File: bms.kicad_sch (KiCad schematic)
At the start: 36 parts, among them IC1 BQ25303JRTER, J1 10118192-0002LF, J4 691213710002, J4 Conn_01x01_Pin, J5 Conn_01x01_Pin, U1 TPS63001DRCR, U5 ADP1109AN-12, U6 ADP1109AN-12, U8 MIC2876-5.0YMT-TR

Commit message: routing
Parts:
- 1uH1: footprint VLS252012HBX-1R0M-1:IND_VLS252012HBX-1R0M-1 -> 1 uH Ind:IND_VLS252012HBX-1R0M-1
- C14, C15, C19, C20: footprint (none) -> Capacitor_SMD:C_0603_1608Metric_Pad1.08x0.95mm_HandSolder
- D1: footprint 0603 LED:LEDC1608X35N -> 0603 LED:LED_150060GS75000_WRE-M
- IC1: footprint bq2530rter:RTE0016C -> BQ2530:RTE0016C_NV
- J1: footprint Micro USB:AMPHENOL_10118192-0002LF -> Micro USB:AMPHENOL_10118192-0001LF
- J4: footprint 691213710002:691213710002 -> Connector_PinSocket_2.54mm:PinSocket_1x02_P2.54mm_Horizontal
- L1: footprint 1UH -IND:IND_VLS252012HBX-1R0M-1 -> 1 uH Ind:IND_VLS252012HBX-1R0M-1
- L2: footprint 2.2UH-IND:IND_VLS4012ET-2R2M -> 3.3v Power Ind:VLS4012
- L3, L4: footprint (none) -> 12v Power Ind:46473C
- U1: footprint tps63001:DRC0010J -> TPS63001:TPS63002DRCT
- U5, U6: footprint N_8_ADI -> ADP1109:N_8_ADI
- U8: footprint UDFN8_2X2_MCH -> 5v Converter:UDFN8_2X2_MCH-L
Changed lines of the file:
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@@
       (effects (font (size 1.27 1.27)) (justify left))
     )
-    (property "Footprint" "" (at 262.5852 139.7 0)
+    (property "Footprint" "Capacitor_SMD:C_0603_1608Metric_Pad1.08x0.95mm_HandSolder" (at 262.5852 139.7 0)
       (effects (font (size 1.27 1.27)) hide)
     )
@@
       (effects (font (size 1.27 1.27)))
     )
-    (property "Footprint" "1UH -IND:IND_VLS252012HBX-1R0M-1" (at 235.585 30.48 0)
+    (property "Footprint" "1 uH Ind:IND_VLS252012HBX-1R0M-1" (at 235.585 30.48 0)
       (effects (font (size 1.27 1.27)) hide)
     )
@@
       (effects (font (size 1.27 1.27)) (justify left))
     )
-    (property "Footprint" "" (at 177.4952 140.97 0)
+    (property "Footprint" "Capacitor_SMD:C_0603_1608Metric_Pad1.08x0.95mm_HandSolder" (at 177.4952 140.97 0)
       (effects (font (size 1.27 1.27)) hide)
     )
@@
       (effects (font (size 1.27 1.27)) hide)
     )
-    (property "Footprint" "VLS252012HBX-1R0M-1:IND_VLS252012HBX-1R0M-1" (at 46.99 168.91 0)
+    (property "Footprint" "1 uH Ind:IND_VLS252012HBX-1R0M-1" (at 46.99 168.91 0)
       (effects (font (size 1.27 1.27)) (justify bottom) hide)
     )
@@
       (effects (font (size 1.27 1.27)) (justify right))
     )
-    (property "Footprint" "" (at 116.84 119.38 0)
+    (property "Footprint" "12v Power Ind:46473C" (at 116.84 119.38 0)
       (effects (font (size 1.27 1.27)) hide)
     )
@@
       (effects (font (size 1.27 1.27)) (justify left) hide)
     )
-    (property "Footprint" "691213710002:691213710002" (at 77.47 118.11 0)
+    (property "Footprint" "Connector_PinSocket_2.54mm:PinSocket_1x02_P2.54mm_Horizontal" (at 77.47 118.11 0)
       (effects (font (size 1.27 1.27)) (justify bottom) hide)
     )
@@
       (effects (font (size 1.524 1.524)))
     )
-    (property "Footprint" "N_8_ADI" (at 234.95 133.35 0)
+    (property "Footprint" "ADP1109:N_8_ADI" (at 234.95 133.35 0)
       (effects (font (size 1.27 1.27) italic) hide)
     )
@@
       (effects (font (size 1.27 1.27)))
     )
-    (property "Footprint" "bq2530rter:RTE0016C" (at 234.95 44.45 0)
+    (property "Footprint" "BQ2530:RTE0016C_NV" (at 234.95 44.45 0)
       (effects (font (size 1.27 1.27)) (justify left) hide)
     )
@@
       (effects (font (size 0.254 0.254)))
     )
-    (property "Footprint" "0603 LED:LEDC1608X35N" (at 200.025 63.5 0)
+    (property "Footprint" "0603 LED:LED_150060GS75000_WRE-M" (at 200.025 63.5 0)
       (effects (font (size 1.27 1.27)) (justify bottom) hide)
     )
@@
       (effects (font (size 1.27 1.27)) hide)
     )
-    (property "Footprint" "Micro USB:AMPHENOL_10118192-0002LF" (at 29.21 123.19 0)
+    (property "Footprint" "Micro USB:AMPHENOL_10118192-0001LF" (at 29.21 123.19 0)
       (effects (font (size 1.27 1.27)) (justify bottom) hide)
     )
@@
       (effects (font (size 1.27 1.27)) (justify right))
     )
-    (property "Footprint" "" (at 201.93 118.11 0)
+    (property "Footprint" "12v Power Ind:46473C" (at 201.93 118.11 0)
       (effects (font (size 1.27 1.27)) hide)
     )
@@
       (effects (font (size 1.27 1.27)) (justify left))
     )
-    (property "Footprint" "" (at 129.2352 184.15 0)
+    (property "Footprint" "Capacitor_SMD:C_0603_1608Metric_Pad1.08x0.95mm_HandSolder" (at 129.2352 184.15 0)
       (effects (font (size 1.27 1.27)) hide)
     )
@@
       (effects (font (size 1.524 1.524)))
     )
-    (property "Footprint" "UDFN8_2X2_MCH" (at 59.69 173.99 0)
+    (property "Footprint" "5v Converter:UDFN8_2X2_MCH-L" (at 59.69 173.99 0)
       (effects (font (size 1.27 1.27) italic) hide)
     )
@@
       (effects (font (size 1.524 1.524)))
     )
-    (property "Footprint" "tps63001:DRC0010J" (at 63.5 63.5 0)
+    (property "Footprint" "TPS63001:TPS63002DRCT" (at 63.5 63.5 0)
       (effects (font (size 1.27 1.27) italic) hide)
     )
@@
       (effects (font (size 1.524 1.524)))
     )
-    (property "Footprint" "N_8_ADI" (at 149.86 134.62 0)
+    (property "Footprint" "ADP1109:N_8_ADI" (at 149.86 134.62 0)
       (effects (font (size 1.27 1.27) italic) hide)
     )
@@
       (effects (font (size 1.27 1.27)))
     )
-    (property "Footprint" "2.2UH-IND:IND_VLS4012ET-2R2M" (at 62.865 35.56 0)
+    (property "Footprint" "3.3v Power Ind:VLS4012" (at 62.865 35.56 0)
       (effects (font (size 1.27 1.27)) hide)
     )
@@
       (effects (font (size 1.27 1.27)) (justify right))
     )
-    (property "Footprint" "" (at 33.3248 179.07 0)
-      (effects (font (size 1.27 1.27)) hide)
-    )
+    (property "Footprint" "Capacitor_SMD:C_0603_1608Metric_Pad1.08x0.95mm_HandSolder" (at 33.3248 179.07 0)
+      (effects (font (size 1.27 1.27)) hide)
+    )

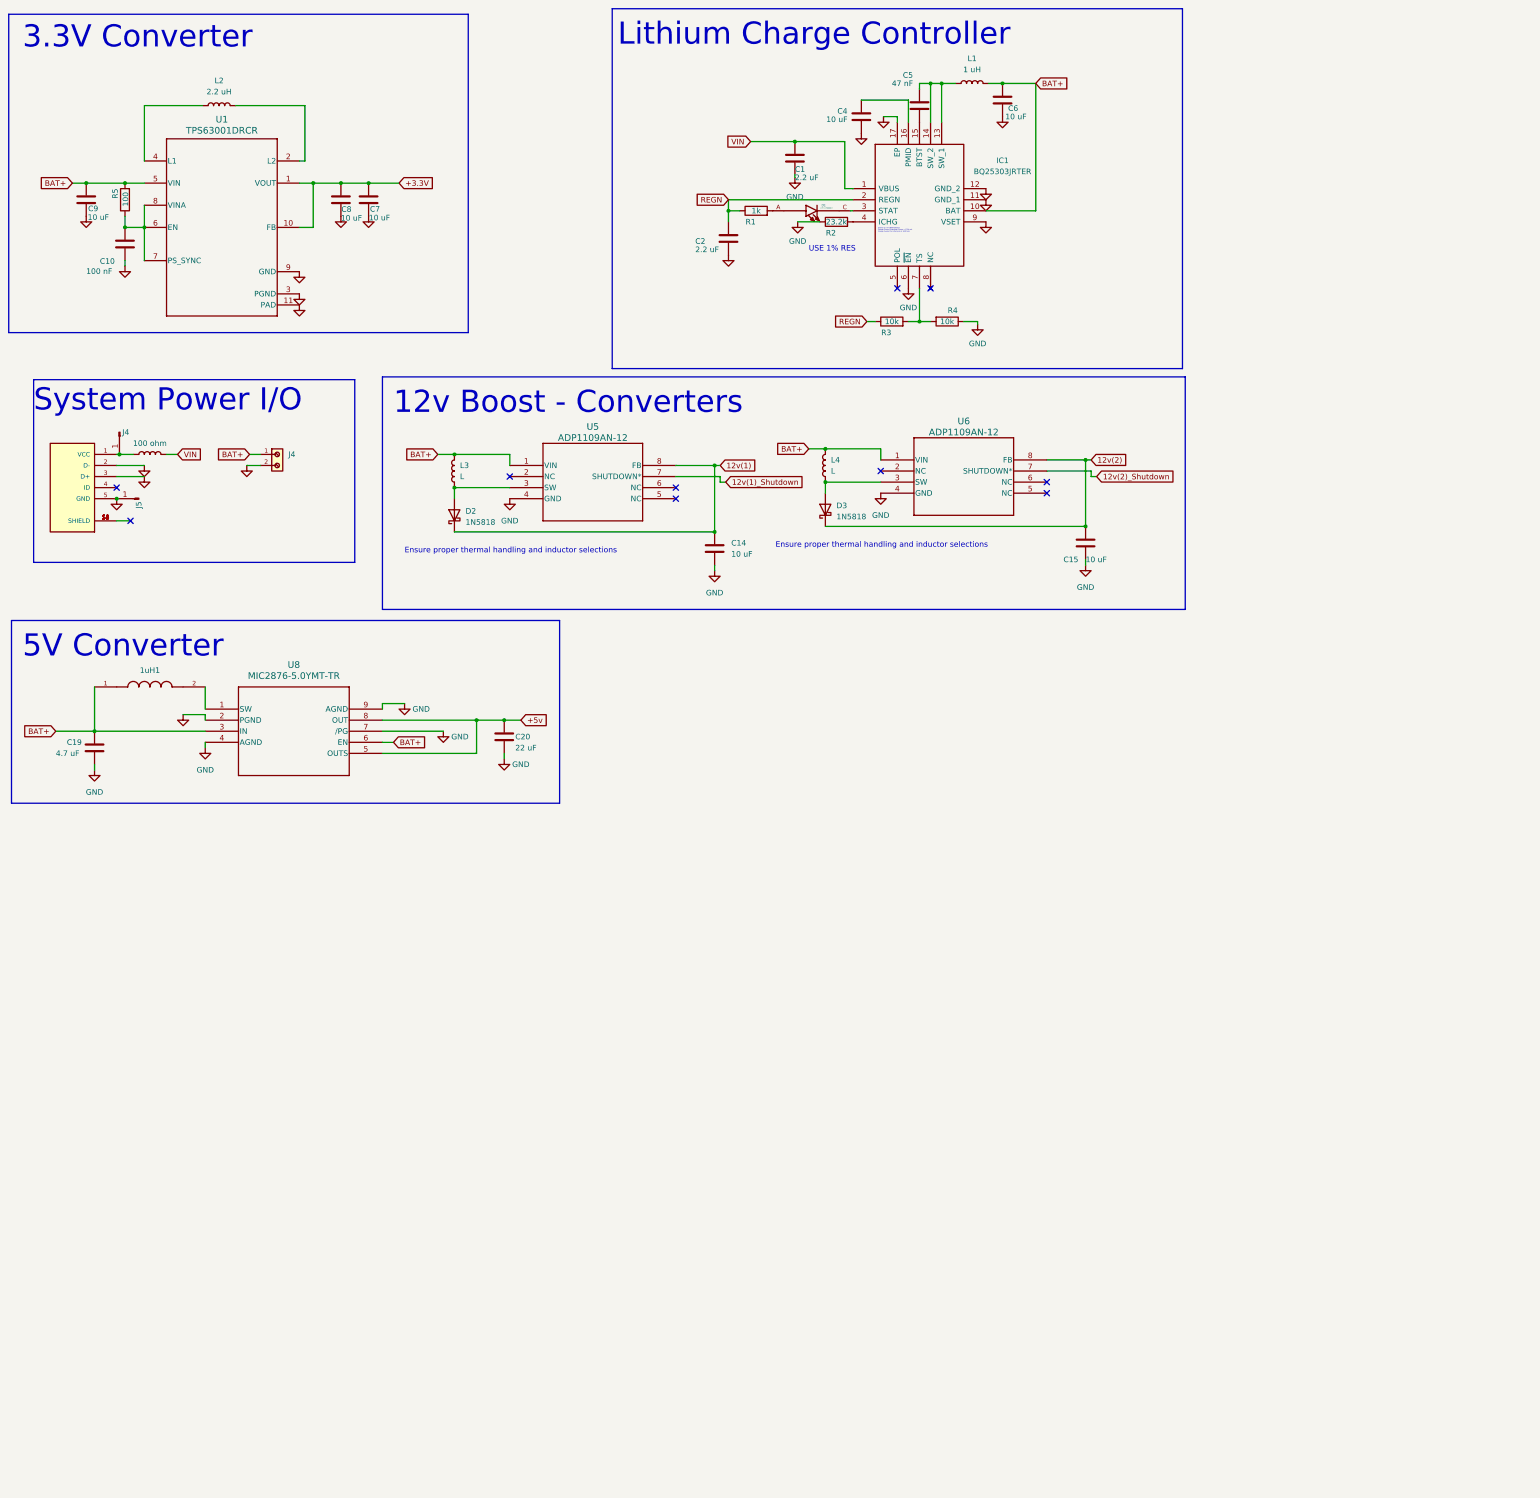
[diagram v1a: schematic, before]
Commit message: Routing begin
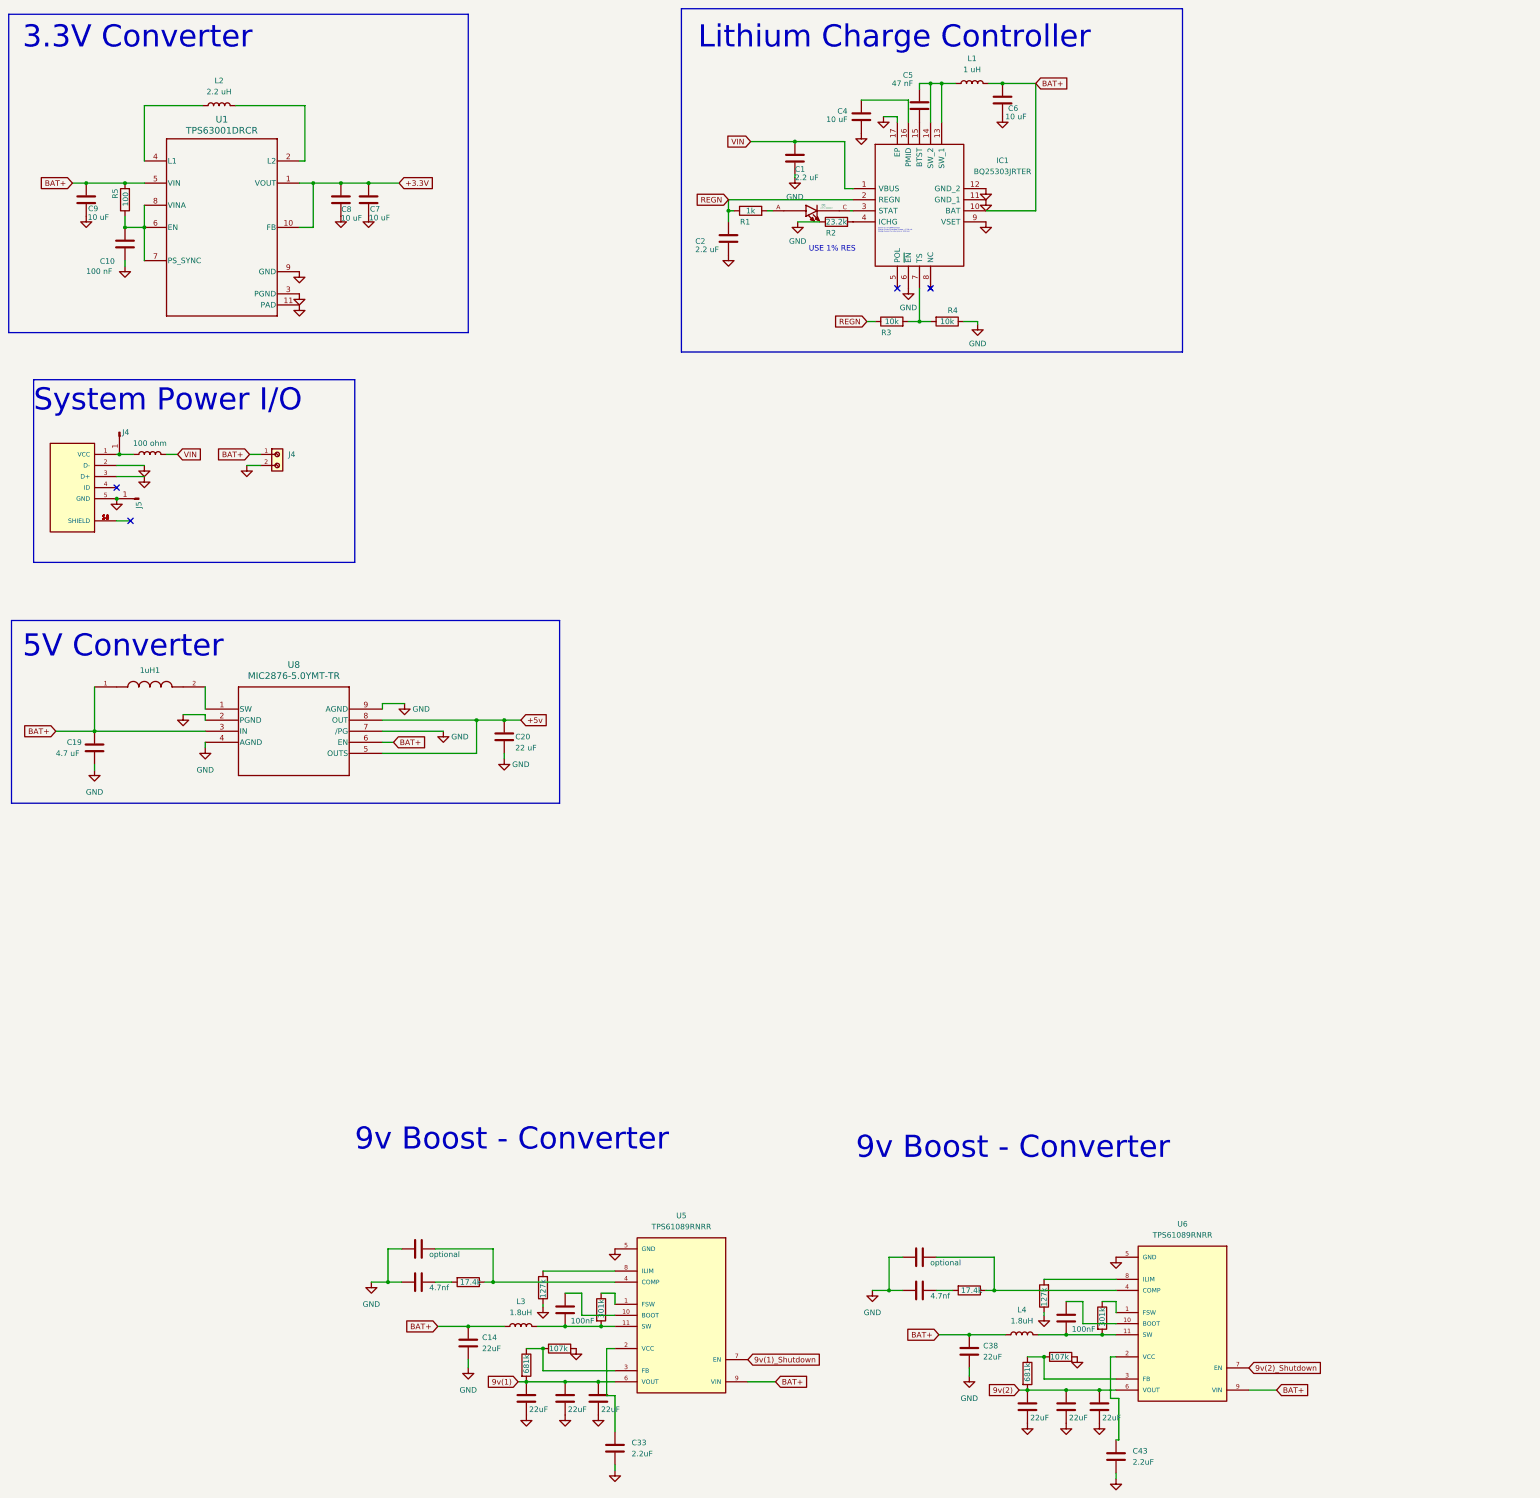
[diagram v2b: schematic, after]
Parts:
- removed D2, D3: 1N5818, Diode_THT:D_DO-41_SOD81_P10.16mm_Horizontal, symbol Diode:1N5818
- removed U5, U6: ADP1109AN-12, ADP1109:N_8_ADI, symbol ADP1109:ADP1109AN-12
- added C30, C31, C32, C38, C39, C41, C42: 22uF, Capacitor_SMD:C_0603_1608Metric_Pad1.08x0.95mm_HandSolder, symbol Device:C
- added C33, C43: 2.2uF, Capacitor_SMD:C_0603_1608Metric_Pad1.08x0.95mm_HandSolder, symbol Device:C
- added C34, C37: 4.7nf, Capacitor_SMD:C_0603_1608Metric_Pad1.08x0.95mm_HandSolder, symbol Device:C
- added C35, C36: optional, Capacitor_SMD:C_0603_1608Metric_Pad1.08x0.95mm_HandSolder, symbol Device:C
- added C40: 100nF, Capacitor_SMD:C_0603_1608Metric_Pad1.08x0.95mm_HandSolder, symbol Device:C
- added R19, R28: 301k, Resistor_SMD:R_0603_1608Metric_Pad0.98x0.95mm_HandSolder, symbol Device:R
- added R20, R25: 681k, Resistor_SMD:R_0603_1608Metric_Pad0.98x0.95mm_HandSolder, symbol Device:R
- added R21, R27: 107k, Resistor_SMD:R_0603_1608Metric_Pad0.98x0.95mm_HandSolder, symbol Device:R
- added R22, R26: 127k, Resistor_SMD:R_0603_1608Metric_Pad0.98x0.95mm_HandSolder, symbol Device:R
- added R23, R24: 17.4k, Resistor_SMD:R_0603_1608Metric_Pad0.98x0.95mm_HandSolder, symbol Device:R
- added U5, U6: TPS61089RNRR, TPS61089:IC_TPS61089RNRR, symbol TPS61089:TPS61089RNRR
- C14: value 10 uF -> 22uF
- C15: value 10 uF -> 100nF
- L3, L4: value L -> 1.8uH; footprint 12v Power Ind:46473C -> 9V_Power_IND:IND_7030-WE-LHMI_WRE-L
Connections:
- net 12v(1) is gone; now on net BAT+: C14.1
- net BAT+: now also L3.1, L4.1, C38.1, U5.9 (VIN), U6.9 (VIN); no longer L3.2, L4.2
- net GND: now also C30.2, C31.2, C32.2, C33.2, C34.1, C35.1, C36.1, C37.1, C38.2, C39.2, C41.2, C42.2, C43.2, R21.2, R22.1, R26.1, R27.2, U5.5 (GND), U6.5 (GND); no longer C15.2
- net 12v(2): no longer names the net of C15.1
- net 12v(2): now also U5.10 (BOOT)
- new net: C15.2, L3.2, R19.2, U5.11 (SW)
- new net: R26.2, U6.8 (ILIM)
- new net: R25.1, R27.1, U6.3 (FB)
- new net: C34.2, R23.2
- new net: R19.1, U5.1 (FSW)
- new net: C33.1, U5.2 (VCC)
- new net: R20.1, R21.1, U5.3 (FB)
- new net: C35.2, R23.1, U5.4 (COMP)
- new net: R22.2, U5.8 (ILIM)
- new net: C36.2, R24.1, U6.4 (COMP)
- new net: C37.2, R24.2
- new net: C43.1, U6.2 (VCC)
- new net: C40.2, L4.2, R28.2, U6.11 (SW)
- new net: R28.1, U6.1 (FSW)
- new net: C40.1, U6.10 (BOOT)
- new net 9v(1): C30.1, C31.1, C32.1, R20.2, U5.6 (VOUT)
- new net 9v(1)_Shutdown: U5.7 (EN)
- new net 9v(2): C39.1, C41.1, C42.1, R25.2, U6.6 (VOUT)
- new net 9v(2)_Shutdown: U6.7 (EN)
- no-connect marks 10 -> 4
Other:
- note added: "9v Boost - Converter"
- note removed: "12v Boost - Converters"
- note removed: "Ensure proper thermal handling and inductor selections"
- moved on the sheet: R1

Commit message: Tedi Check dis over pls.
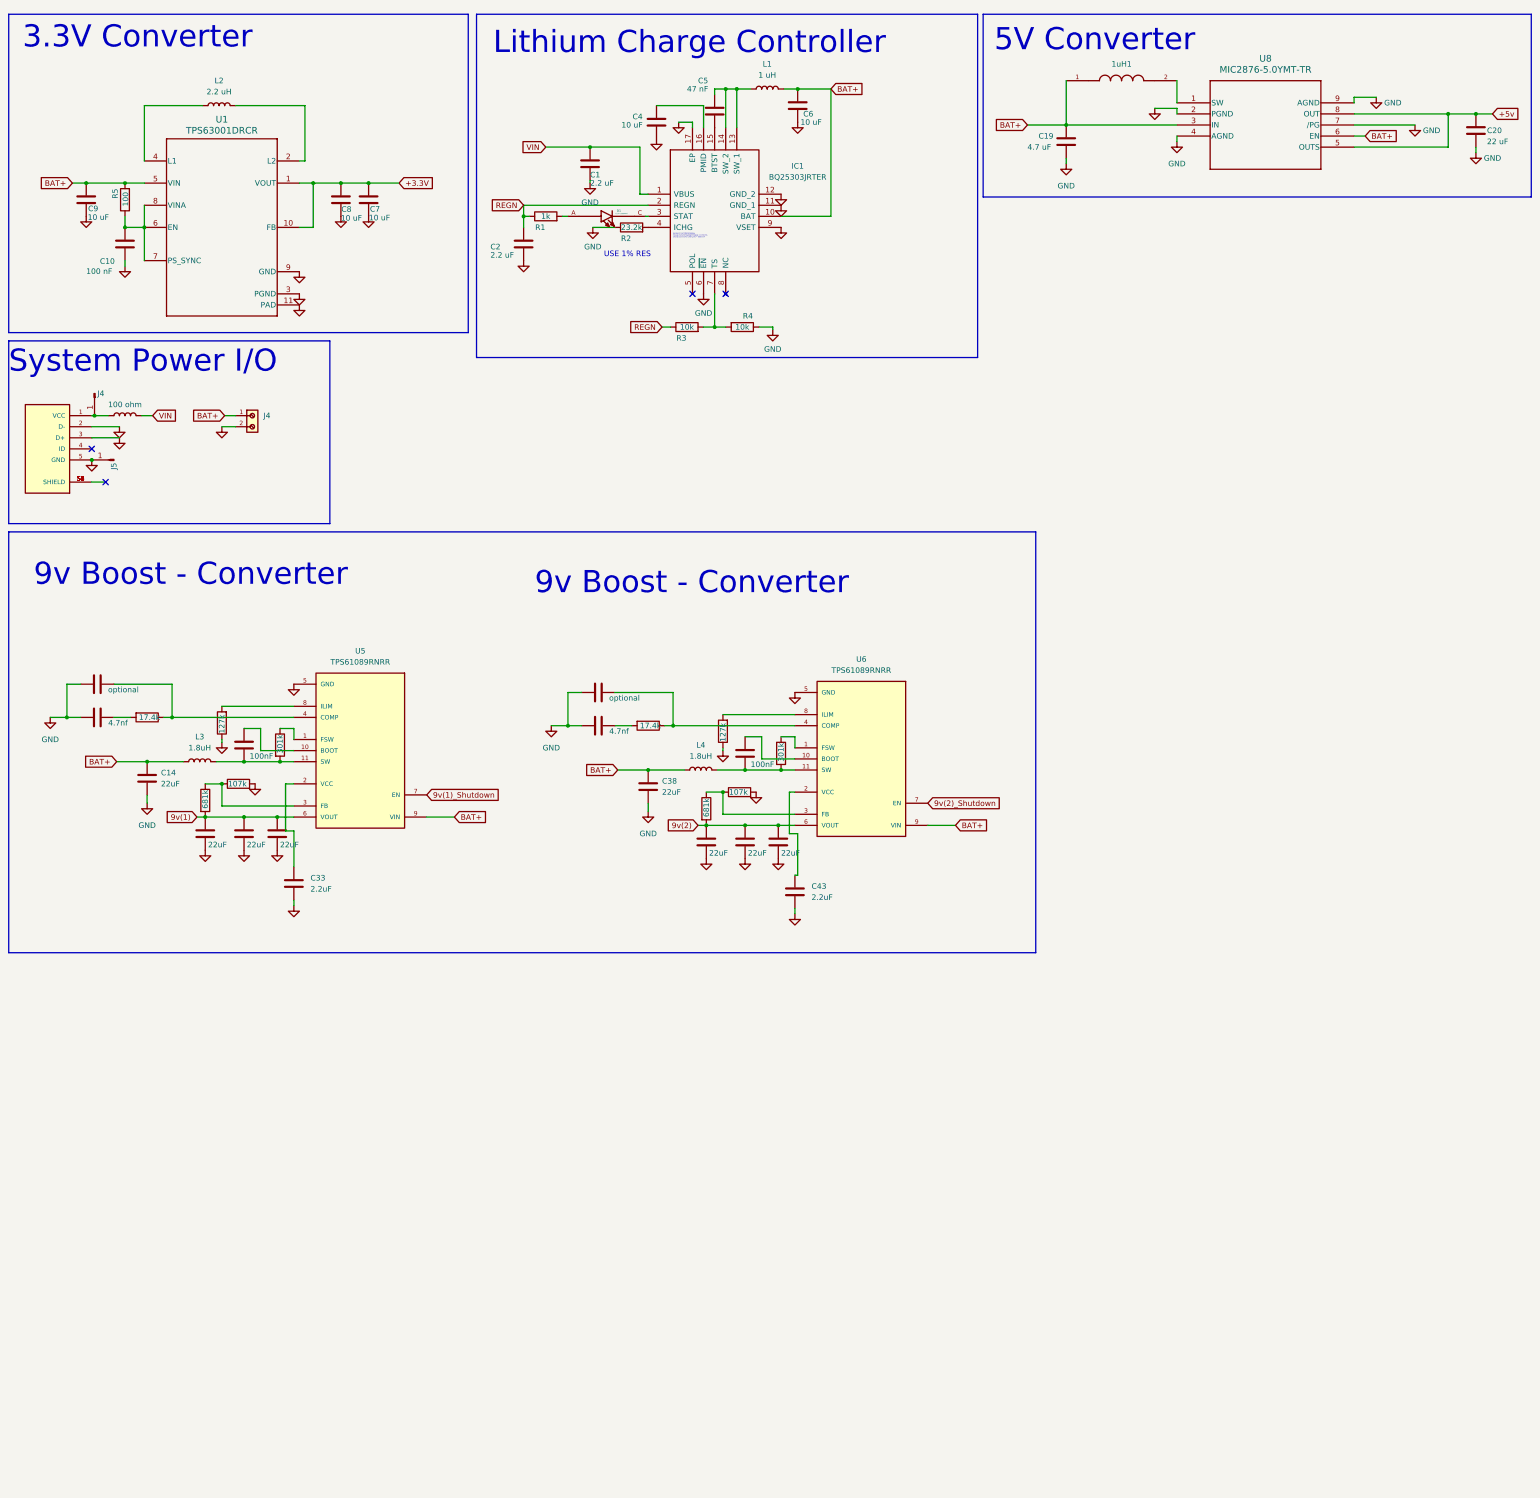
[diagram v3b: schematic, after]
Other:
- moved on the sheet: 1uH1, C1, C14, C19, C2, C20, C33, C38, C4, C43, C5, C6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
